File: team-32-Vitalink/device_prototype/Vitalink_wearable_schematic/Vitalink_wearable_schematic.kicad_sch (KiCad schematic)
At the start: 8 parts, among them J1 USB_C_Receptacle_PowerOnly_24P, U1 ESP32-C6-MINI-1, U2 LSM6DS3, U4 MAX6005, U5 Si7020-A20

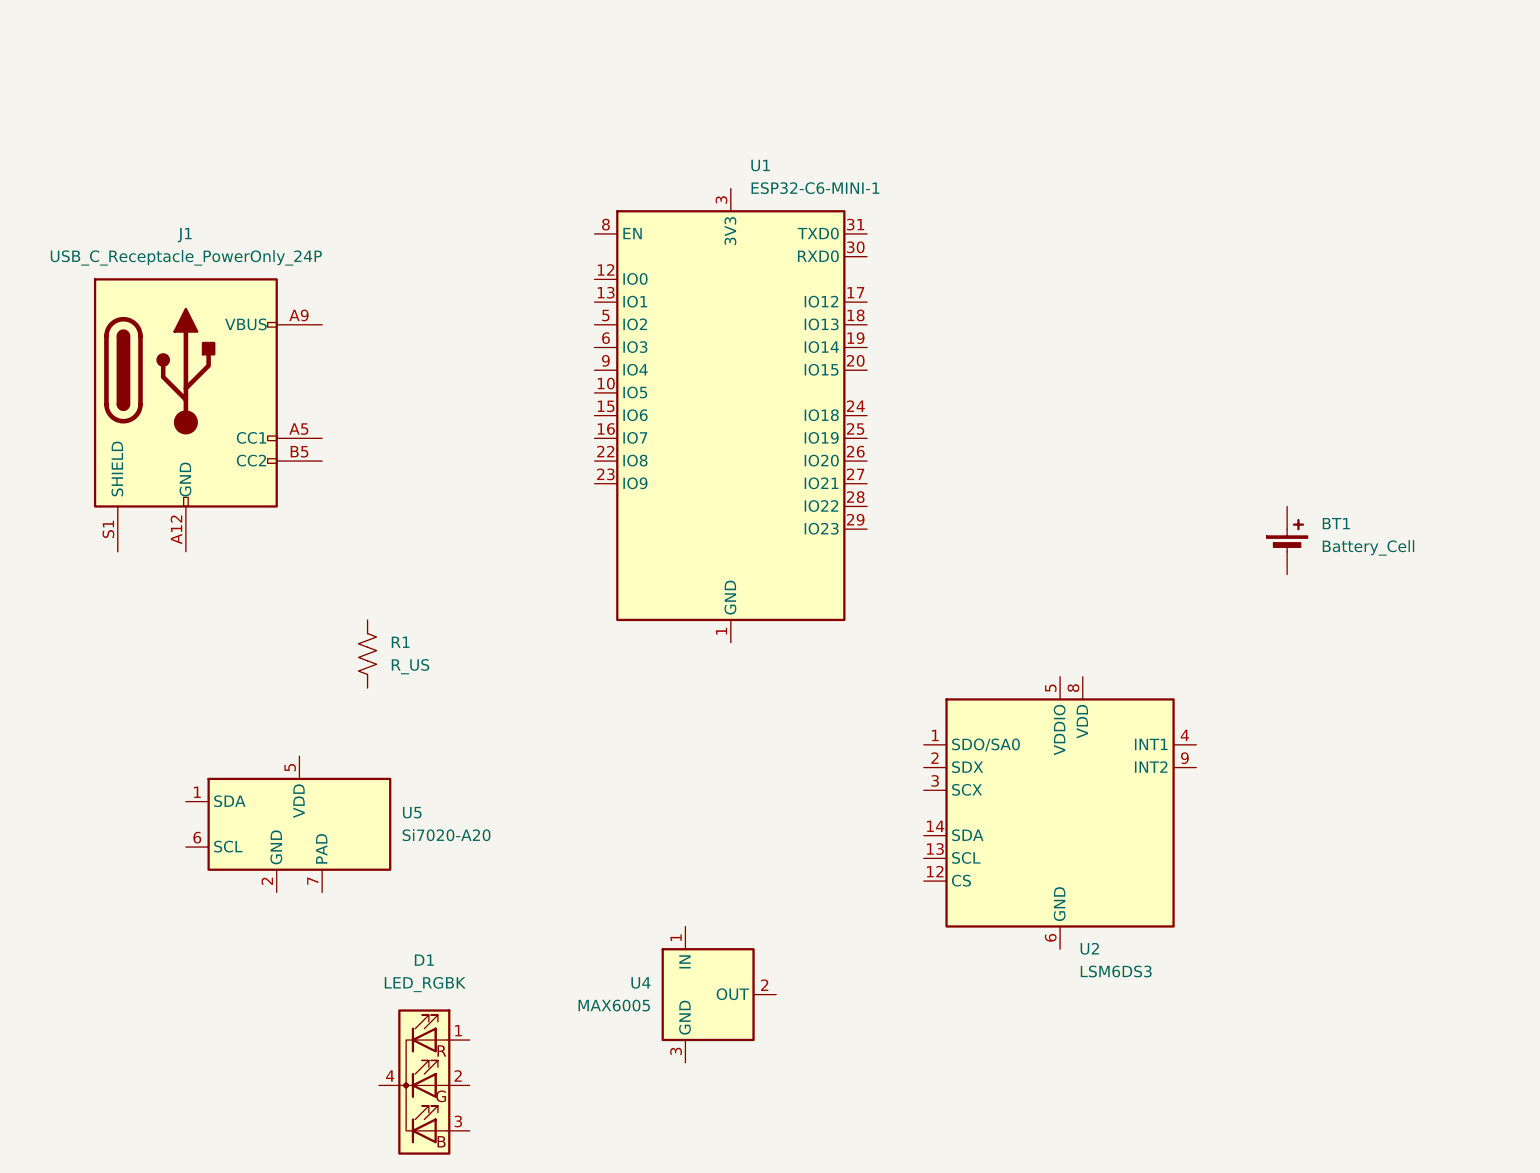
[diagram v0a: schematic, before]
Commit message: finished the schematic design
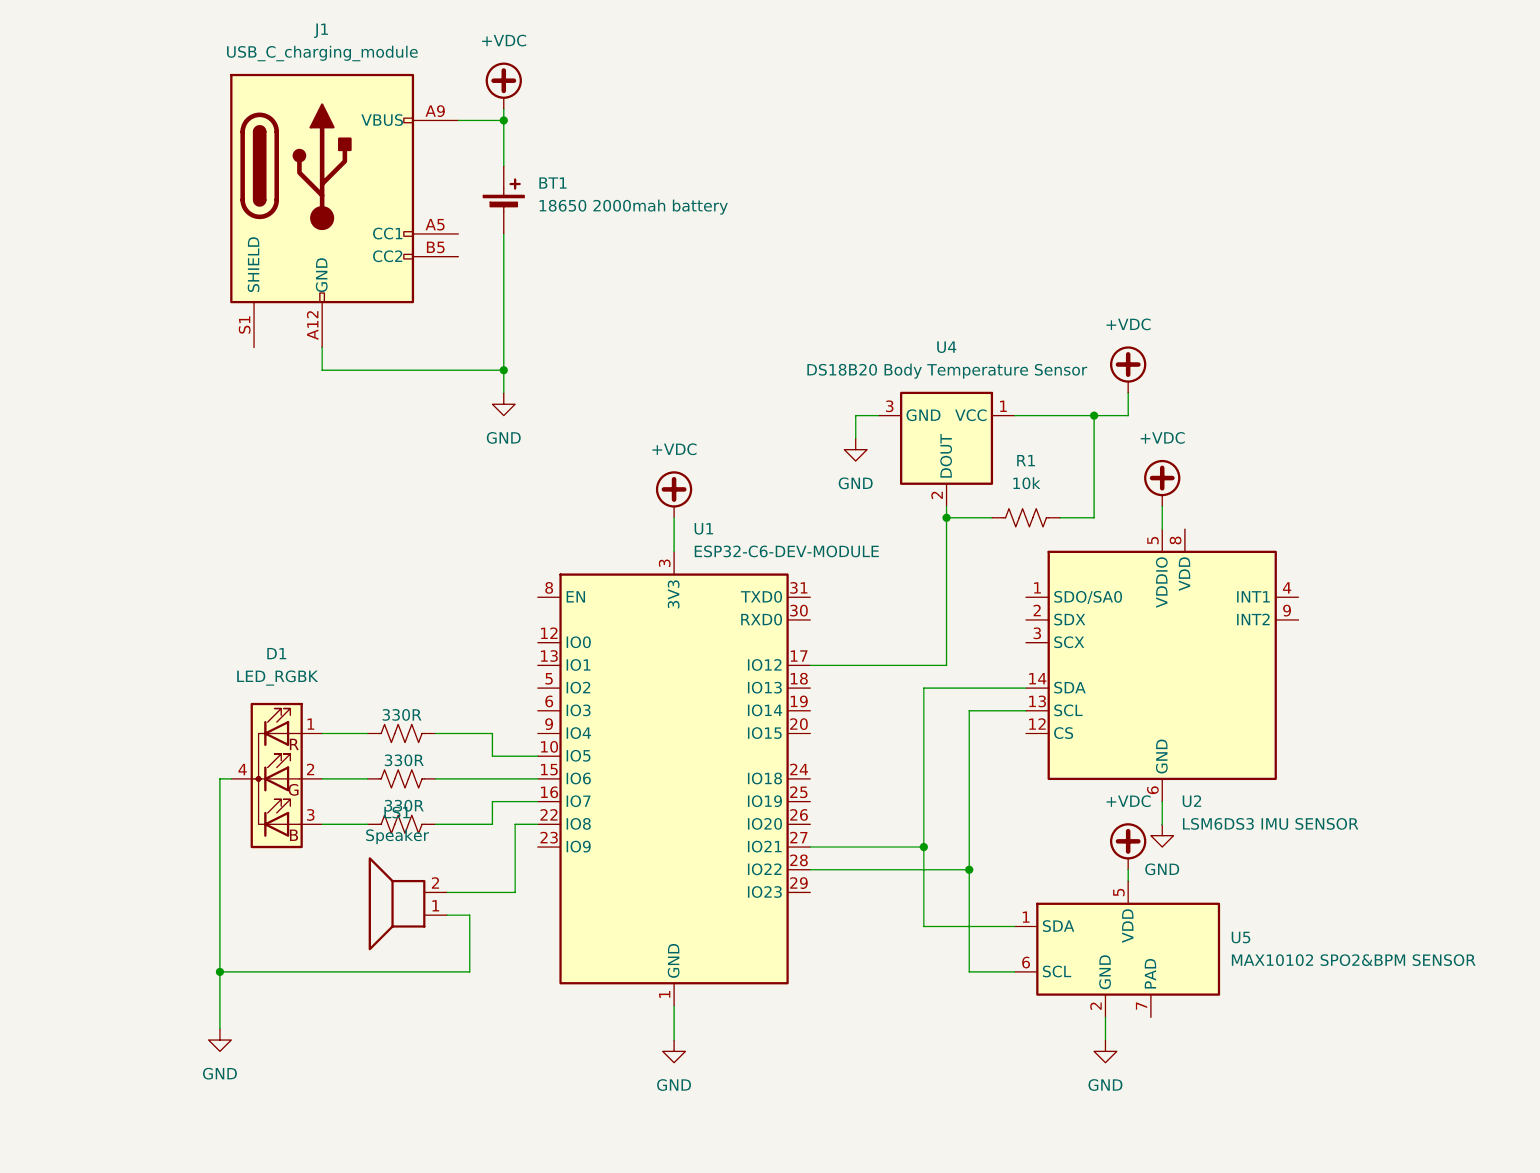
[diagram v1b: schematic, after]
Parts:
- added LS1: Speaker, symbol Device:Speaker
- added R2, R3, R4: 330R, symbol Device:R_US
- BT1: value Battery_Cell -> 18650 2000mah battery
- J1: value USB_C_Receptacle_PowerOnly_24P -> USB_C_charging_module
- R1: value R_US -> 10k
- U1: value ESP32-C6-MINI-1 -> ESP32-C6-DEV-MODULE
- U2: value LSM6DS3 -> LSM6DS3 IMU SENSOR
- U4: value MAX6005 -> DS18B20 Body Temperature Sensor
- U5: value Si7020-A20 -> MAX10102 SPO2&BPM SENSOR
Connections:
- net at D1.1 (RA): now also R2.2
- net at D1.2 (GA): now also R3.2
- net at D1.3 (BA): now also R4.2
- net GND: now reaches D1.4 (K)
- net GND: now also BT1.2 (-), J1.A1 (GND), J1.A12 (GND), J1.B1 (GND), J1.B12 (GND), U1.1 (GND), U1.11 (GND), U1.14 (GND), U1.2 (GND), U1.36 (GND), U1.37 (GND), U1.38 (GND), U1.39 (GND), U1.40 (GND), U1.41 (GND), U1.42 (GND), U1.43 (GND), U1.44 (GND), U1.45 (GND), U1.46 (GND), U1.47 (GND), U1.48 (GND), U1.49 (GND), U1.50 (GND), U1.51 (GND), U1.52 (GND), U1.53 (GND), U2.6 (GND), U2.7 (GND), U4.3 (GND), U5.2 (GND), LS1.1
- net at U1.10 (IO5): now also R2.1
- net at U1.15 (IO6): now also R3.1
- net at U1.16 (IO7): now also R4.1
- net at U1.17 (IO12): now also R1.2, U4.2 (DOUT)
- net at U1.22 (IO8): now also LS1.2
- net at U1.27 (IO21): now also U2.14 (SDA), U5.1 (SDA)
- net at U1.28 (IO22): now also U2.13 (SCL), U5.6 (SCL)
- net +VDC: now reaches U1.3 (3V3)
- net +VDC: now also BT1.1 (+), J1.A4 (VBUS), J1.A9 (VBUS), J1.B4 (VBUS), J1.B9 (VBUS), R1.1, U2.5 (VDDIO), U4.1 (VCC), U5.5 (VDD)
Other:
- moved on the sheet: BT1, D1, J1, R1, U1, U2, U4, U5
